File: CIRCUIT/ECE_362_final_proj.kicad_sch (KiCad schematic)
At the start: 30 parts, among them J1 Conn_01x01_Pin, J2 Conn_01x01_Pin, J3 Conn_01x28_Socket, J4 Conn_01x28_Socket, SW3 BUTTON_MODE, SW5 BUTTON_CAPTURE, SW6 BUTTON_MODE, U1 TL084

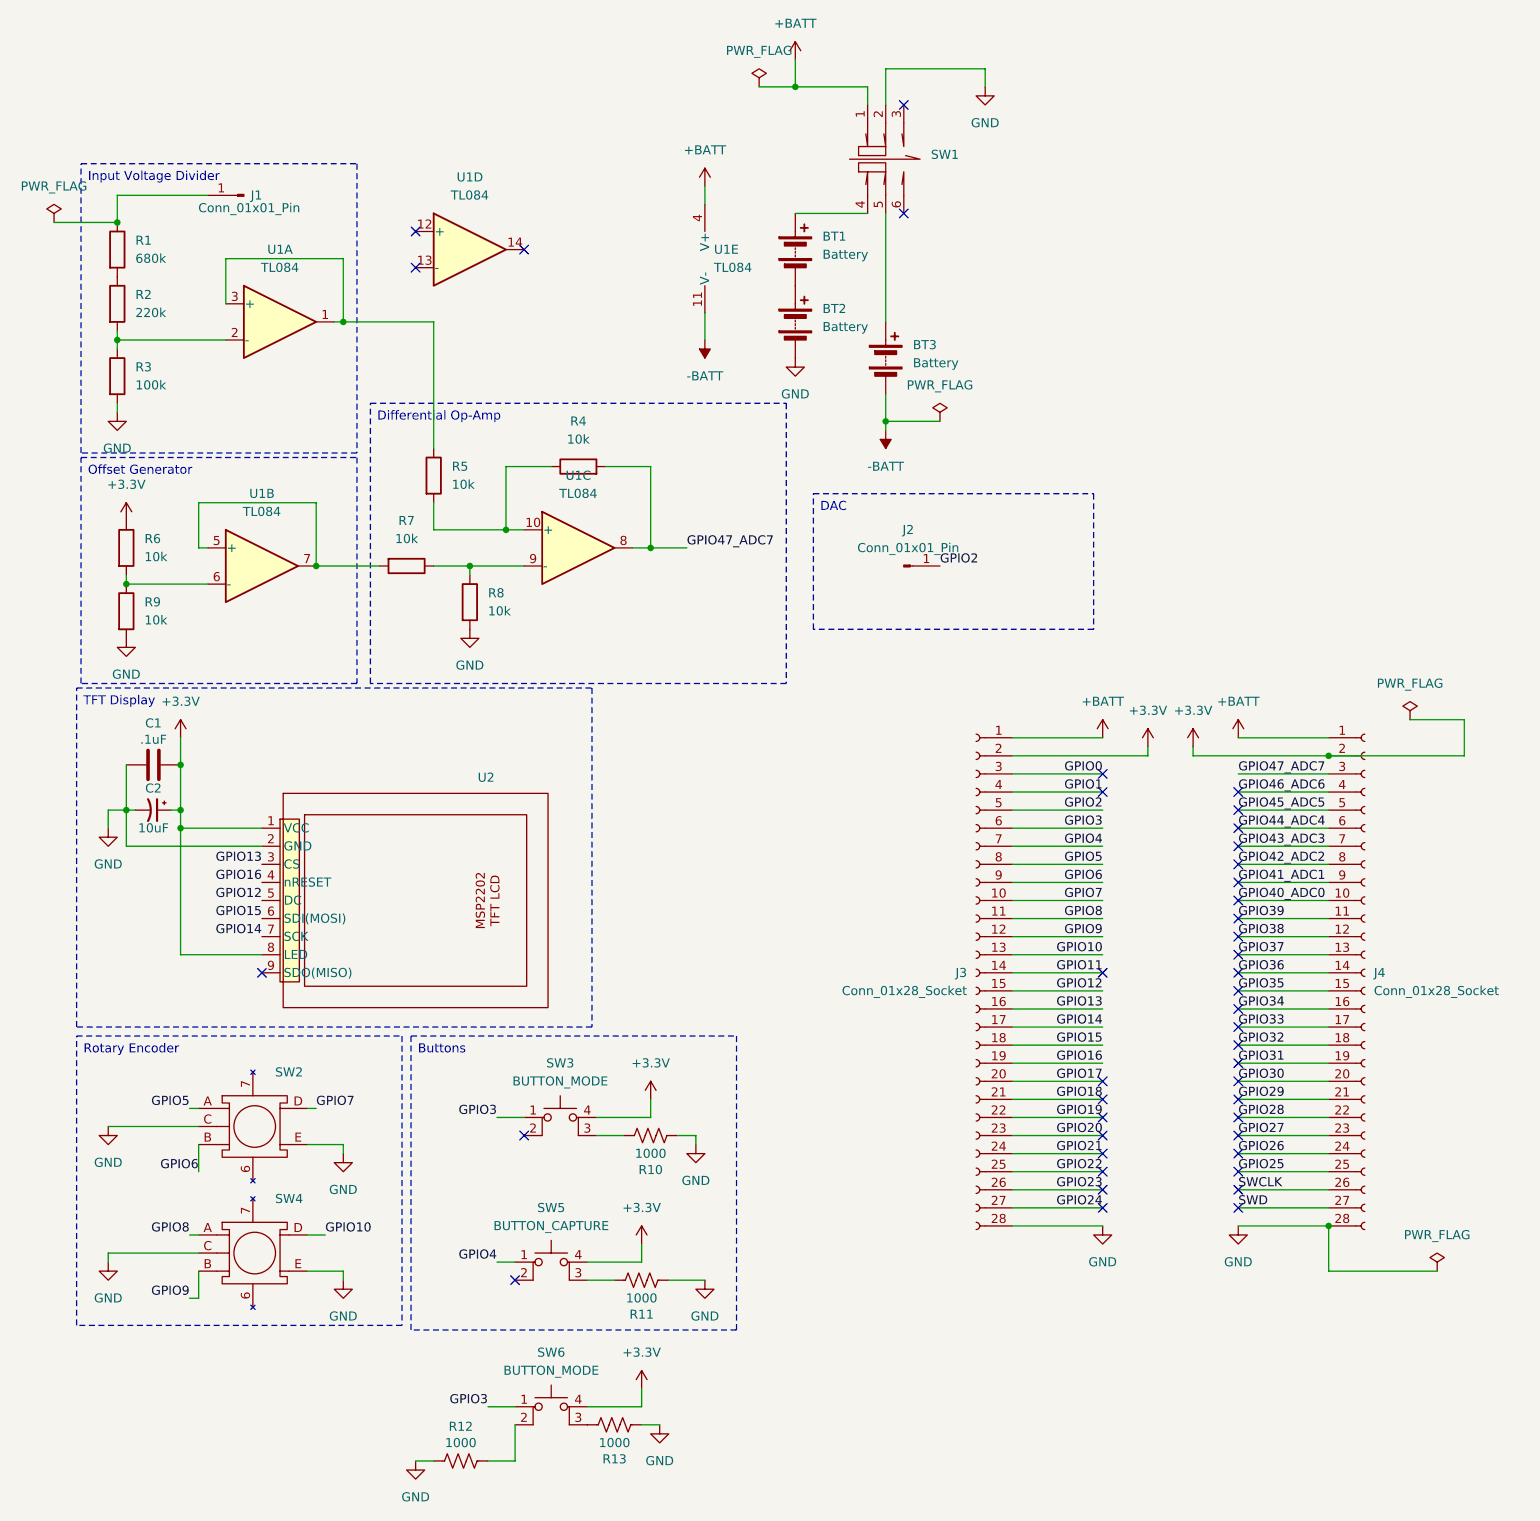
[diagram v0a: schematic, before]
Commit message: final circuit
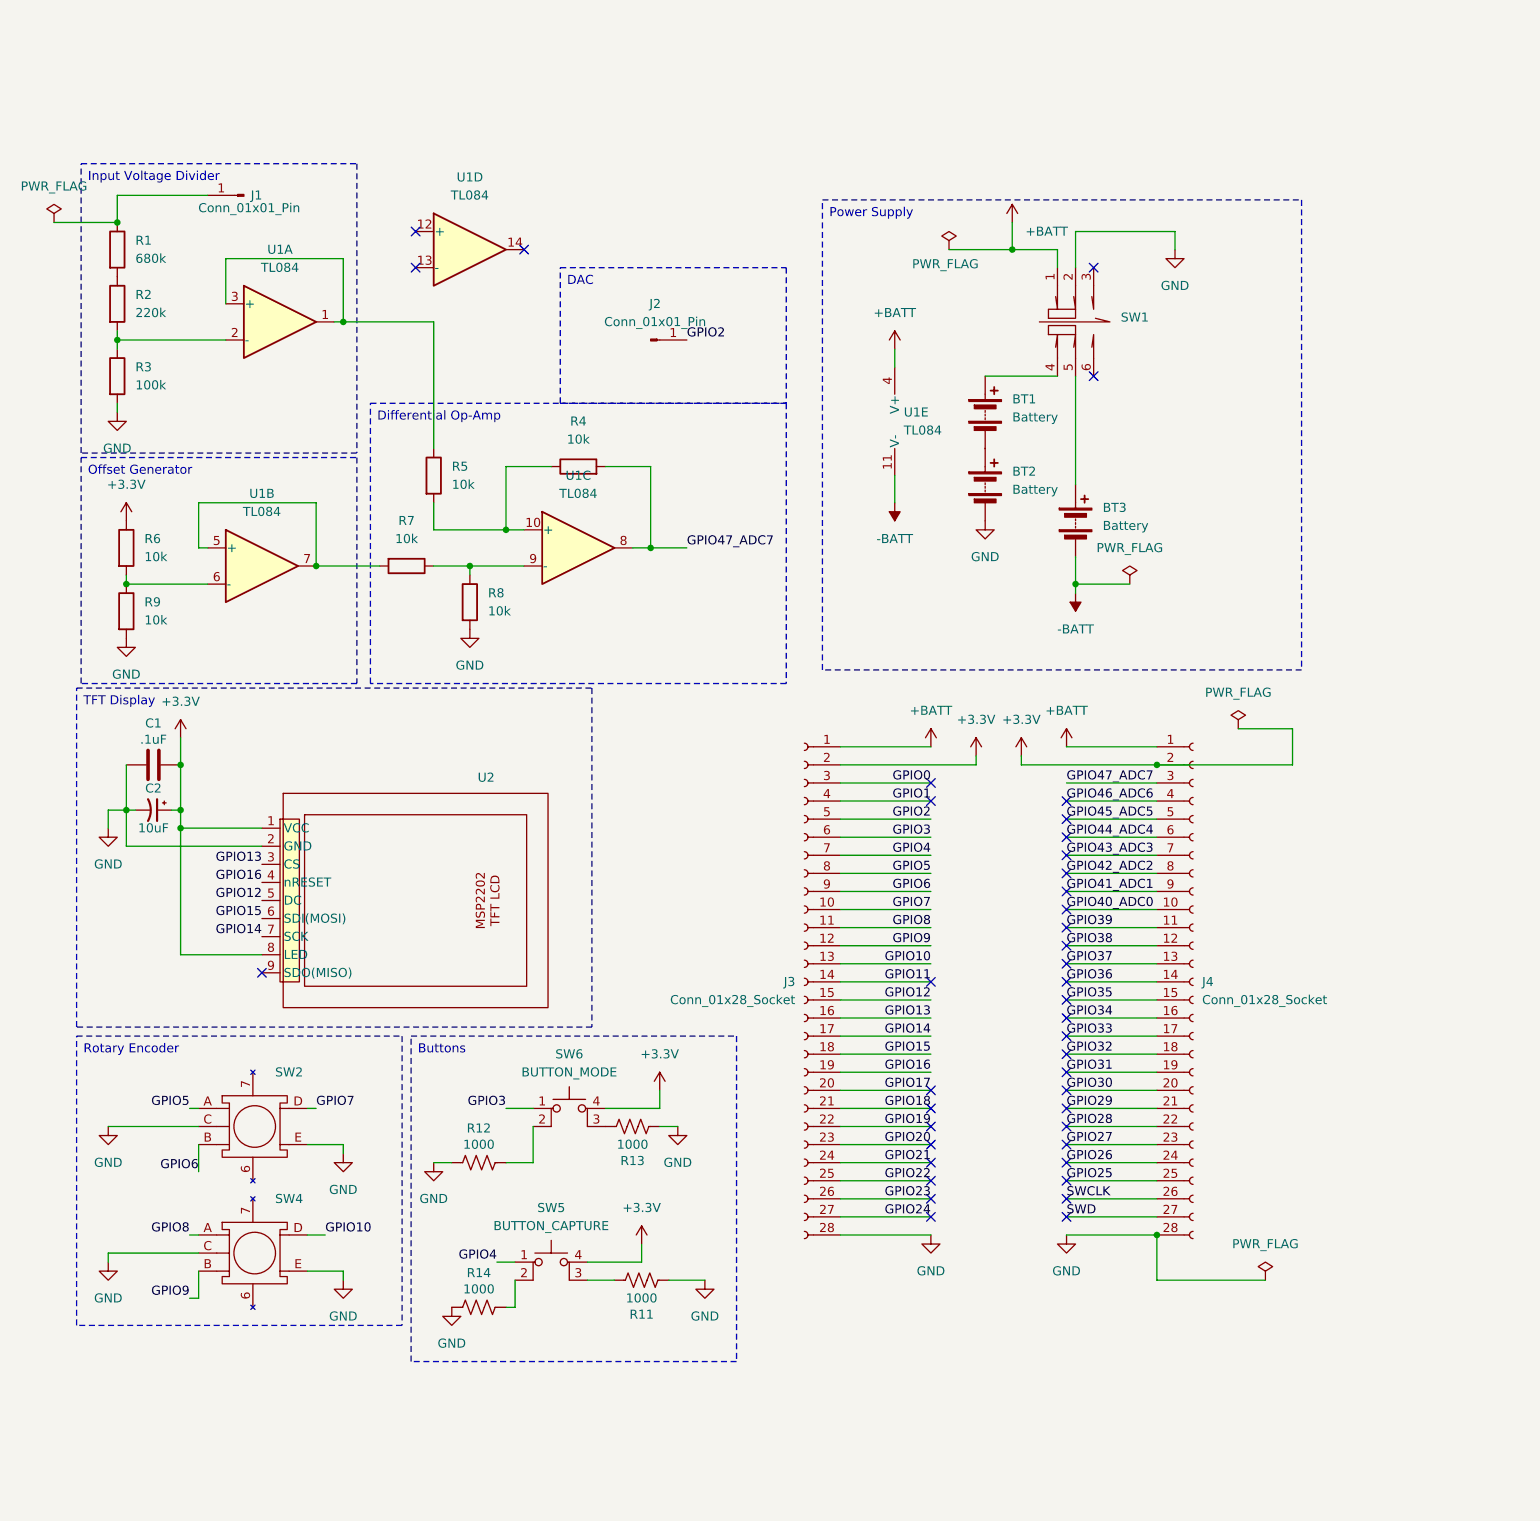
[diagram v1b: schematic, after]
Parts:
- removed R10: 1000, Resistor_SMD:R_0402_1005Metric, symbol Device:R_US
- removed SW3: BUTTON_MODE, Button_Tactile:SW-TH_4P-L6.0-W6.0-P4.50-LS6.5, symbol Switch:SW_MEC_5E
- added R14: 1000, Resistor_SMD:R_0402_1005Metric, symbol Device:R_US
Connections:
- net GND: now also R14.2
- net at SW5.2: now also R14.1
- no-connect marks 43 -> 41
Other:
- moved on the sheet: BT1, BT2, BT3, J2, J3, J4, R12, R13, SW1, SW6, U1E
